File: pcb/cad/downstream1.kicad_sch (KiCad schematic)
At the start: 14 parts, among them J601 USB_C_Receptacle, U601 ECMF02-2AMX6, U602 ECMF02-2AMX6, U603 ECMF02-2AMX6, U604 ECMF02-2AMX6, U605 ECMF02-2AMX6, U606 ECMF02-2AMX6, U607 CBTL02043A, U608 TUSB320, U609 PI3USB221E, U610 LM73100, U611 TPS25947xx

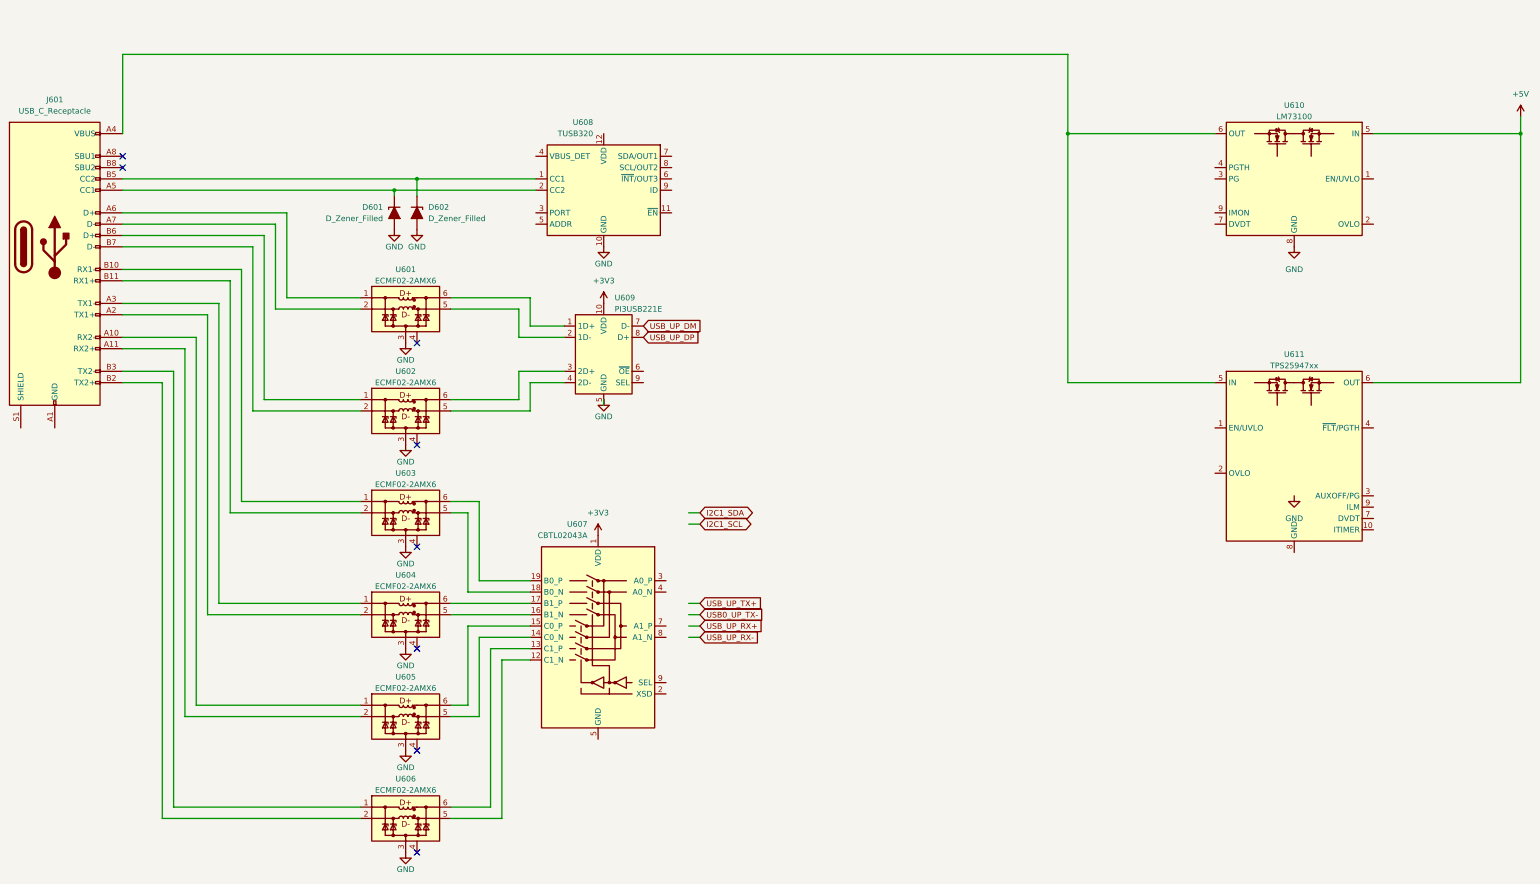
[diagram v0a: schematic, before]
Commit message: moved old-old-old backups and finished preliminary USB architecture
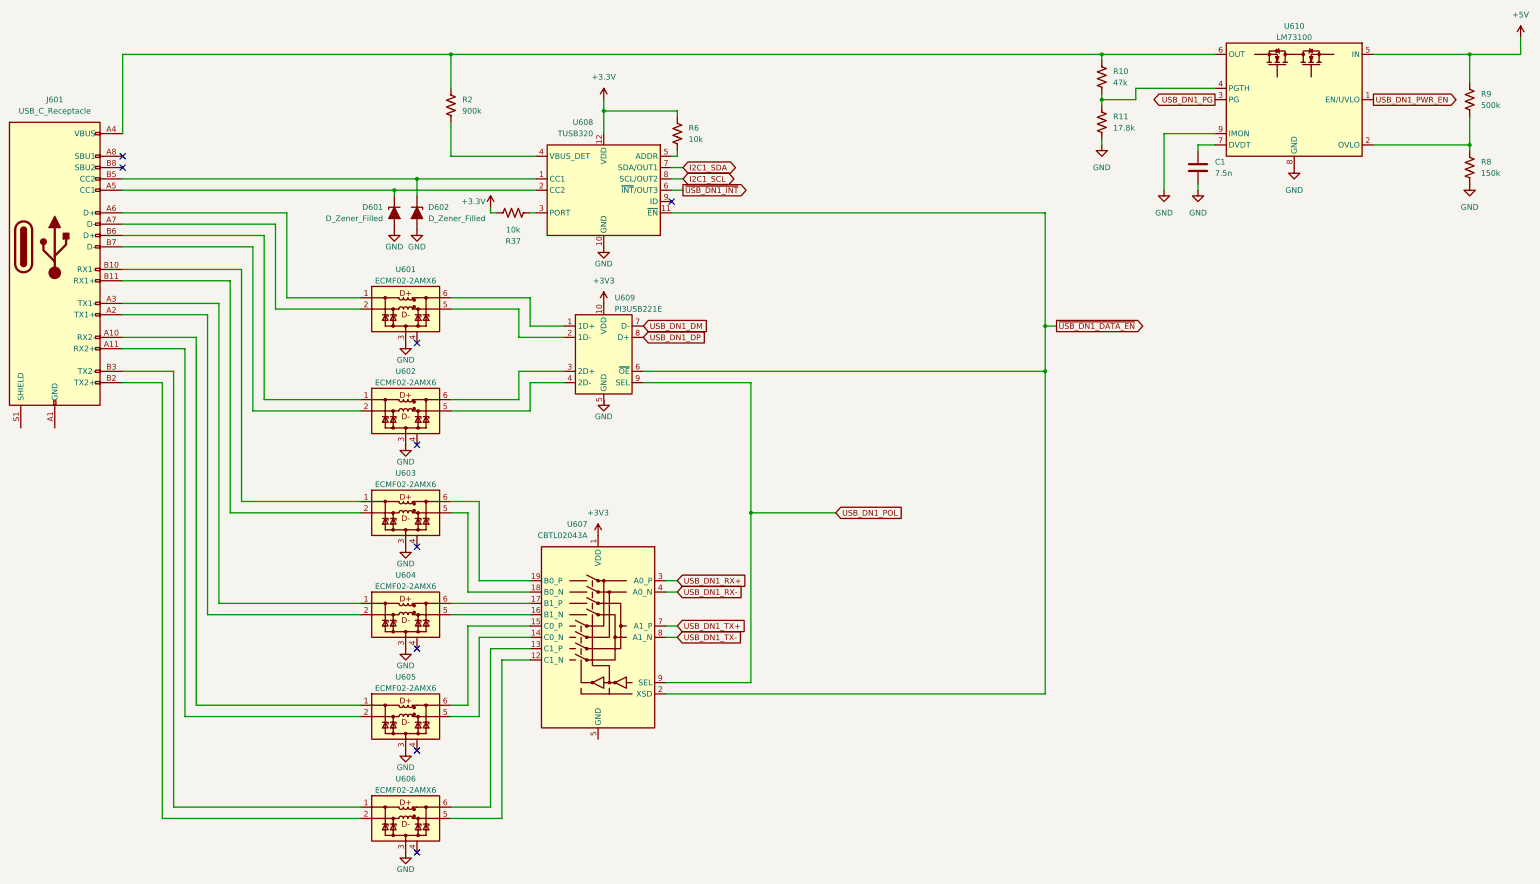
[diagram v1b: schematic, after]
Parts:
- removed U611: TPS25947xx, symbol Library:TI_TPS25947
- added C1: 7.5n, symbol Device:C
- added R10: 47k, symbol Device:R_US
- added R11: 17.8k, symbol Device:R_US
- added R2: 900k, symbol Device:R_US
- added R37, R6: 10k, symbol Device:R_US
- added R8: 150k, symbol Device:R_US
- added R9: 500k, symbol Device:R_US
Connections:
- net +5V: now also R9.1
- net GND: now also U610.9 (IMON), C1.2, R11.2, R8.2
- net I2C1_SCL: now also U608.8 (SCL/OUT2)
- net I2C1_SDA: now also U608.7 (SDA/OUT1)
- net ~{USB_DN1_DATA_EN}: now reaches U607.2 (XSD)
- net ~{USB_DN1_DATA_EN}: now also U608.11 (~{EN}), U609.6 (~{OE})
- net USB_DN1_RX+: now reaches U607.3 (A0_P)
- net USB_DN1_RX-: now reaches U607.4 (A0_N)
- net USB_DN1_TX+: now reaches U607.7 (A1_P)
- net USB_DN1_TX-: now reaches U607.8 (A1_N)
- net USB_DN1_POL: now reaches U607.9 (SEL)
- net USB_DN1_POL: now also U609.9 (SEL)
- net +3.3V: now reaches U608.12 (VDD)
- net +3.3V: now also R37.2, R6.1
- net at U608.3 (PORT): now also R37.1
- net at U608.4 (VBUS_DET): now also R2.2
- net at U608.5 (ADDR): now also R6.2
- net ~{USB_DN1_INT}: now reaches U608.6 (~{INT}/OUT3)
- net at J601.A4 (VBUS), J601.A9 (VBUS), J601.B4 (VBUS)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: now also R10.1, R2.1
- net USB_DN1_PWR_EN: now reaches U610.1 (EN/UVLO)
- net at U610.2 (OVLO): now also R8.1, R9.2
- net USB_DN1_PG: now reaches U610.3 (PG)
- net at U610.4 (PGTH): now also R10.2, R11.1
- net at U610.7 (DVDT): now also C1.1
- net USB_UP_DM renamed USB_DN1_DM
- net USB_UP_DP renamed USB_DN1_DP
- no-connect marks 8 -> 9
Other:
- moved on the sheet: U610
